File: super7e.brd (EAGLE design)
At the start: 135 x 60 mm, 19 parts, among them IC1 STM32F103VCT

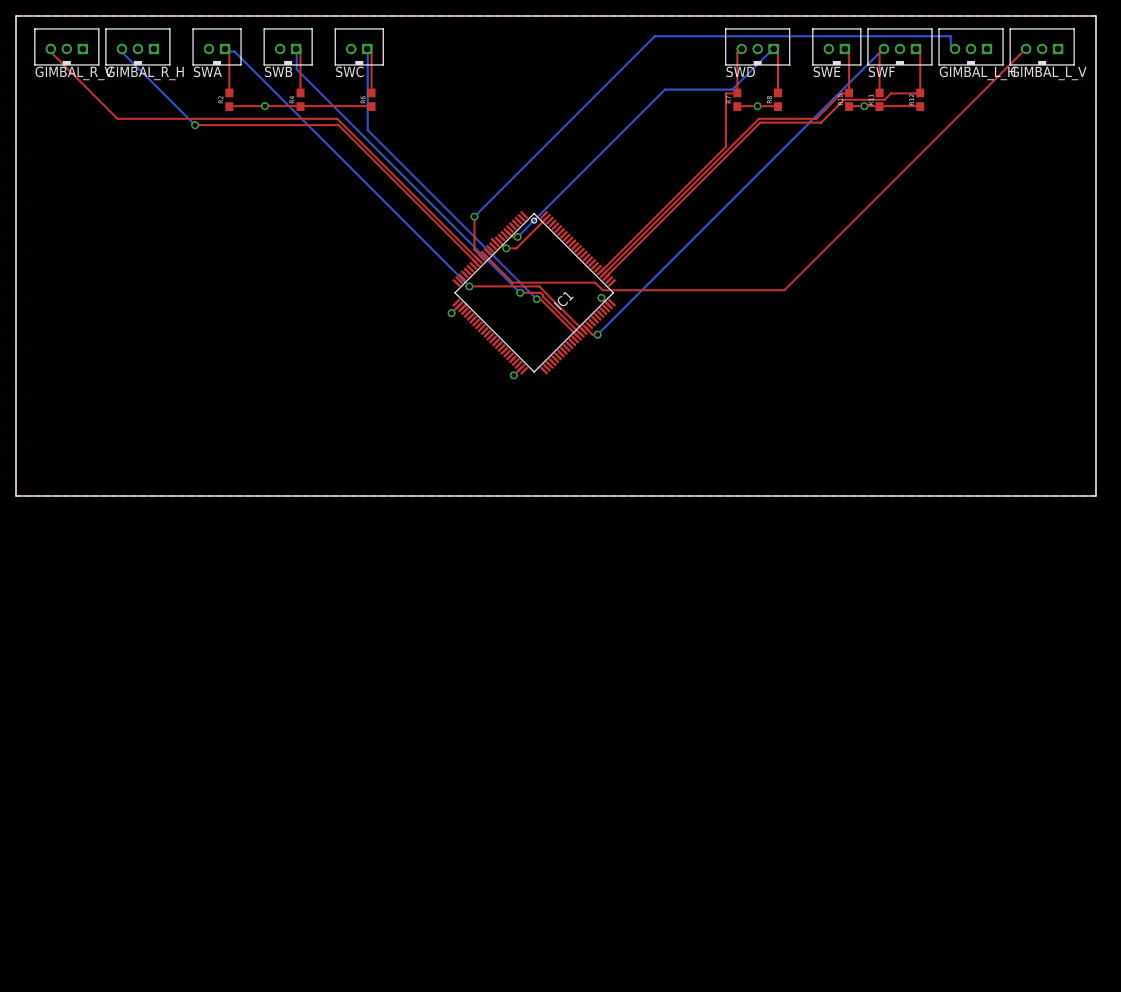
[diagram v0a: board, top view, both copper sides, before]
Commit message: *
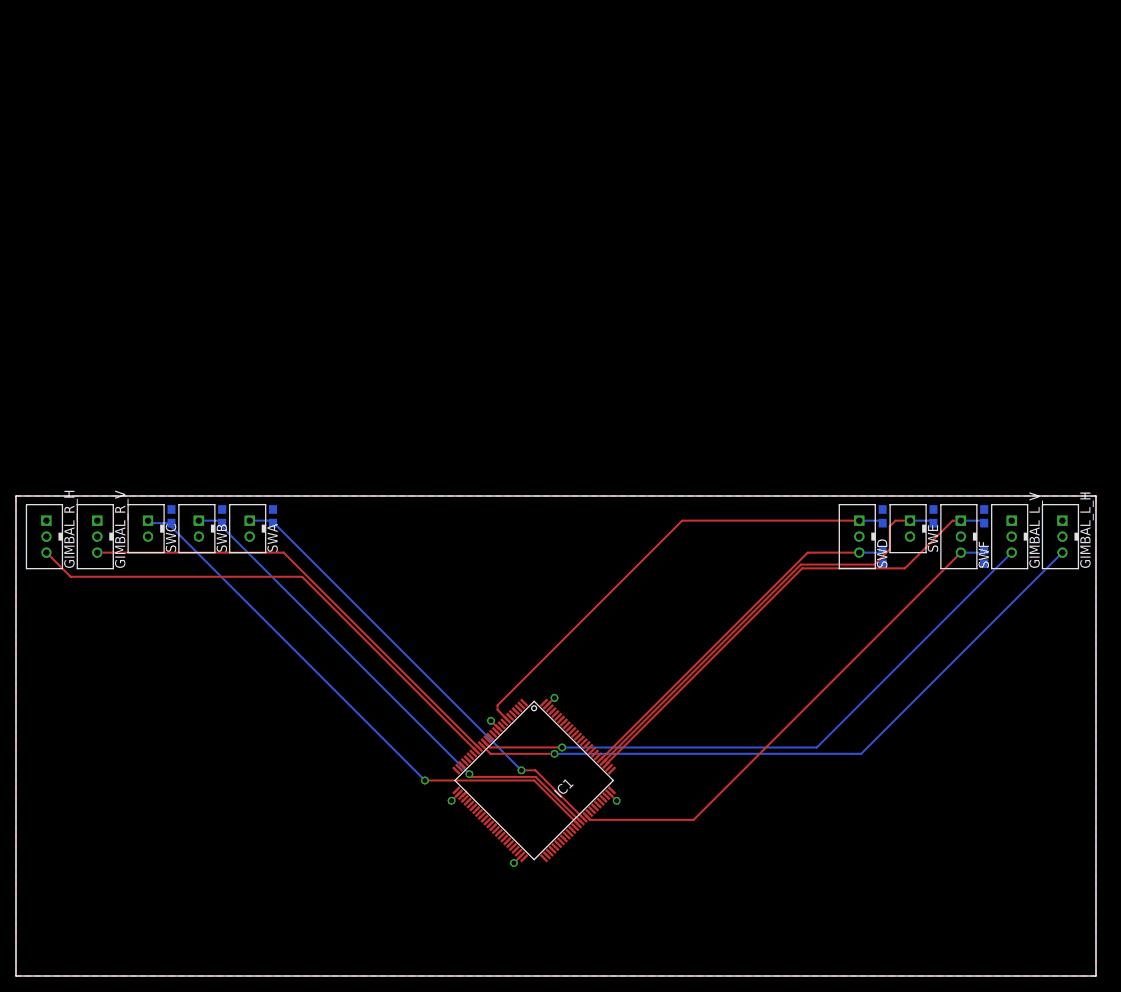
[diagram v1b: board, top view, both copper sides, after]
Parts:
- moved SWC 66.0 mm to (16.5, -5.08), turned to 90 degrees
- moved SWD 62.3 mm to (105.4, -5.08), turned to 90 degrees
- moved GIMBAL_L_H 62.0 mm to (130.8, -5.08), turned to 90 degrees
- moved GIMBAL_R_H 62.0 mm to (3.81, -5.08), turned to 90 degrees
- moved SWB 61.8 mm to (22.9, -5.08), turned to 90 degrees
- moved SWE 61.8 mm to (111.8, -5.08), turned to 90 degrees
- moved SWF 61.4 mm to (118.1, -5.08), turned to 90 degrees
- moved SWA 61.2 mm to (29.2, -5.08), turned to 90 degrees
- moved GIMBAL_L_V 61.1 mm to (124.5, -5.08), turned to 90 degrees
- moved GIMBAL_R_V 61.1 mm to (10.2, -5.08), turned to 90 degrees
- moved IC1 61.0 mm to (64.8, -35.6)
- moved R7 60.0 mm to (108.3, -7.62), flipped to the bottom
- moved R11 58.6 mm to (121.0, -7.62), flipped to the bottom
- moved R6 57.8 mm to (19.4, -2.54), flipped to the bottom, turned to 270 degrees
- moved R8 53.7 mm to (108.3, -2.54), flipped to the bottom, turned to 270 degrees
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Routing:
- net GND: track 44.3 -> 6.76 mm, vias 7 -> 5
- net SW_GEAR: track 53.2 -> 69.7 mm
- net SW_MIX_0: track 49.3 -> 60.2 mm, vias 1 -> 0
- net SW_MIX_2: track 36.0 -> 46.1 mm
- net SW_AIL_DR: track 46.2 -> 55.7 mm
- net SW_RUD_DR: track 65.7 -> 57.2 mm
- net GIMBAL_R_H: track 55.7 -> 64.0 mm, vias 1 -> 0
- net GIMBAL_L_H: track 76.2 -> 83.4 mm
- net GIMBAL_R_V: track 64.7 -> 57.8 mm
- net SW_FMOD_2: track 58.1 -> 64.0 mm, vias 1 -> 0
- net GIMBAL_L_V: track 82.0 -> 76.2 mm, vias 0 -> 1
- net SW_ELE_DR: track 57.9 -> 63.6 mm
- net SW_FMOD_0: track 54.9 -> 60.1 mm
